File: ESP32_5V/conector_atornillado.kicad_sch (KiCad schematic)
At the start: 2 parts, among them J5 Screw_Terminal_01x11, J6 Screw_Terminal_01x11

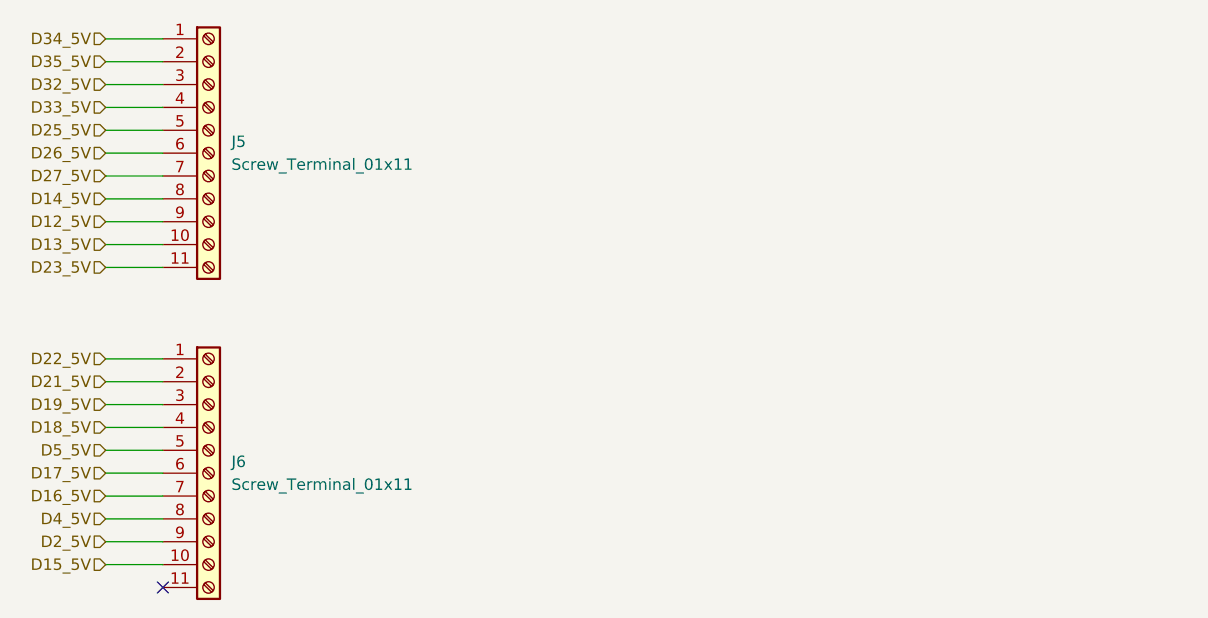
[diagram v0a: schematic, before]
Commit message: update
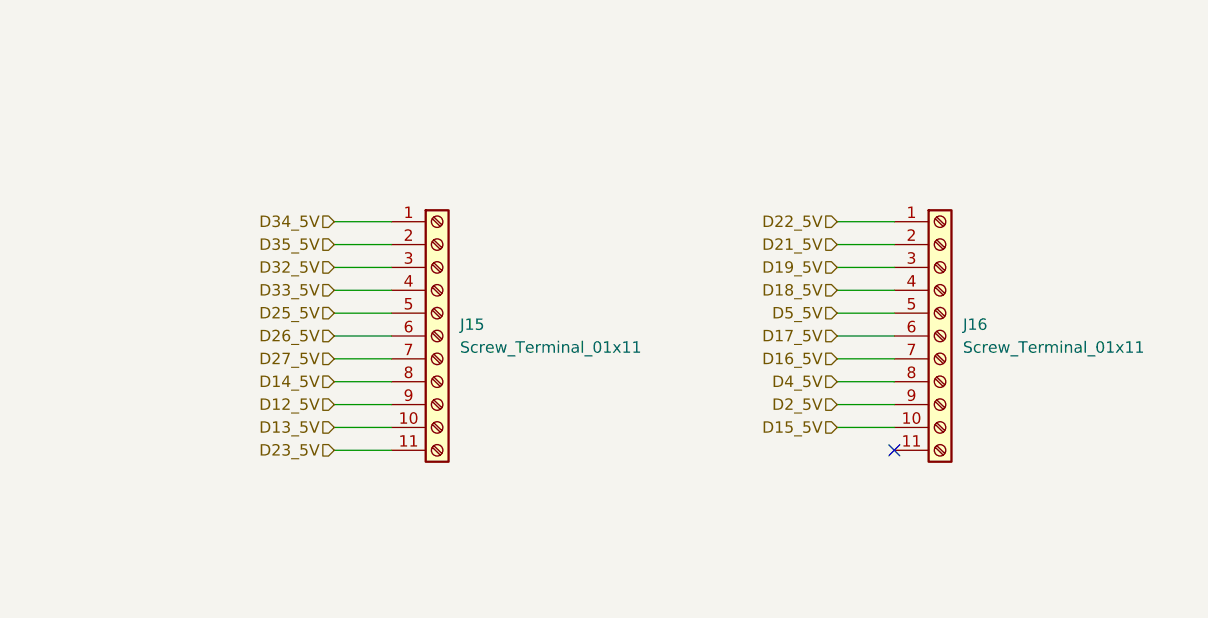
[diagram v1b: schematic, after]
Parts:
- renumbered J5 to J15, J6 to J16
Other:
- moved on the sheet: J15, J16
